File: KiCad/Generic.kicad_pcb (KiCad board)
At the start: 2 copper layers, 19 x 29.1 mm, 13 parts, among them J1 Connector, J2 USB-C, J3 VBUS, M1 D24V5F3-NoSHDN, U1 ESP32-WROOM-32, U2 FT230XQ

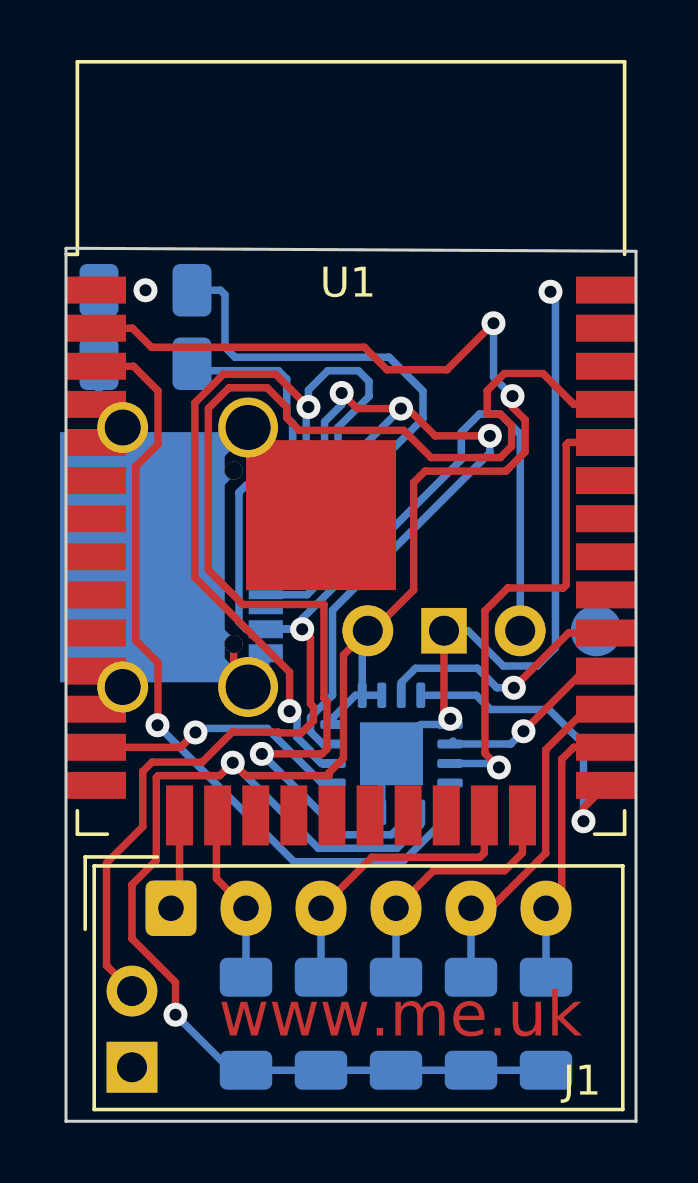
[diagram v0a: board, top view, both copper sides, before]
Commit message: Centred
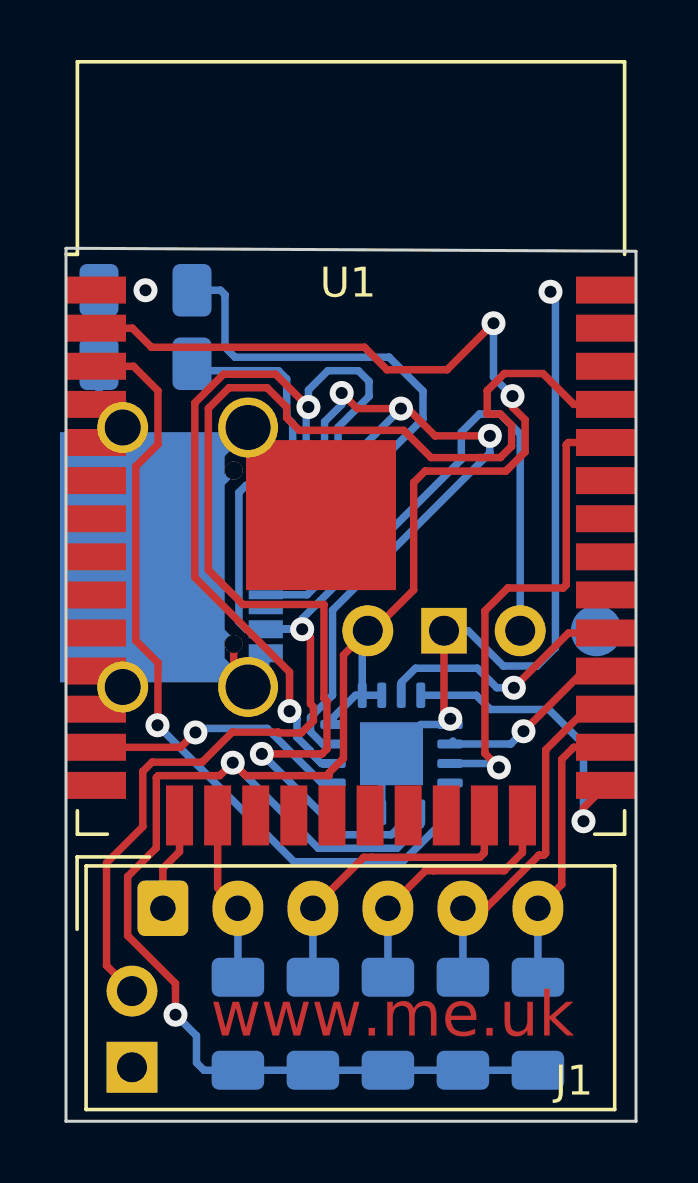
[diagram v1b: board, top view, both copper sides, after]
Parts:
- moved R5 0.27 mm to (128.2, 124.2)
- moved J1 0.27 mm to (115.7, 120.4)
- moved R1 0.27 mm to (118.2, 124.2)
- moved R2 0.27 mm to (120.7, 124.2)
- moved R3 0.27 mm to (123.2, 124.2)
- moved R4 0.27 mm to (125.7, 124.2)
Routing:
- net IO4: track 11.6 -> 12.2 mm
- net IO2: track 9.76 -> 10.4 mm
